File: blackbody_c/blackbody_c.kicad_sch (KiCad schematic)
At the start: 6 parts

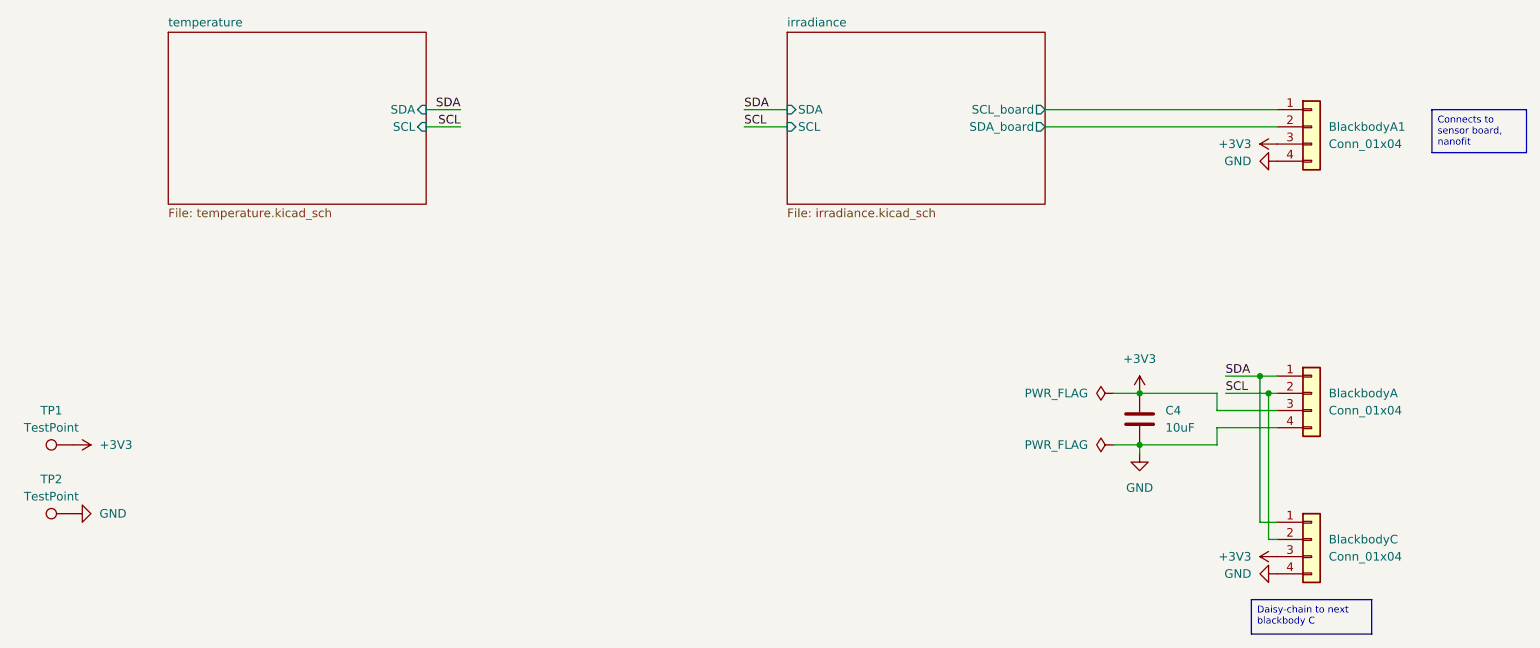
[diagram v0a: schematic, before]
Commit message: layout iteration 1
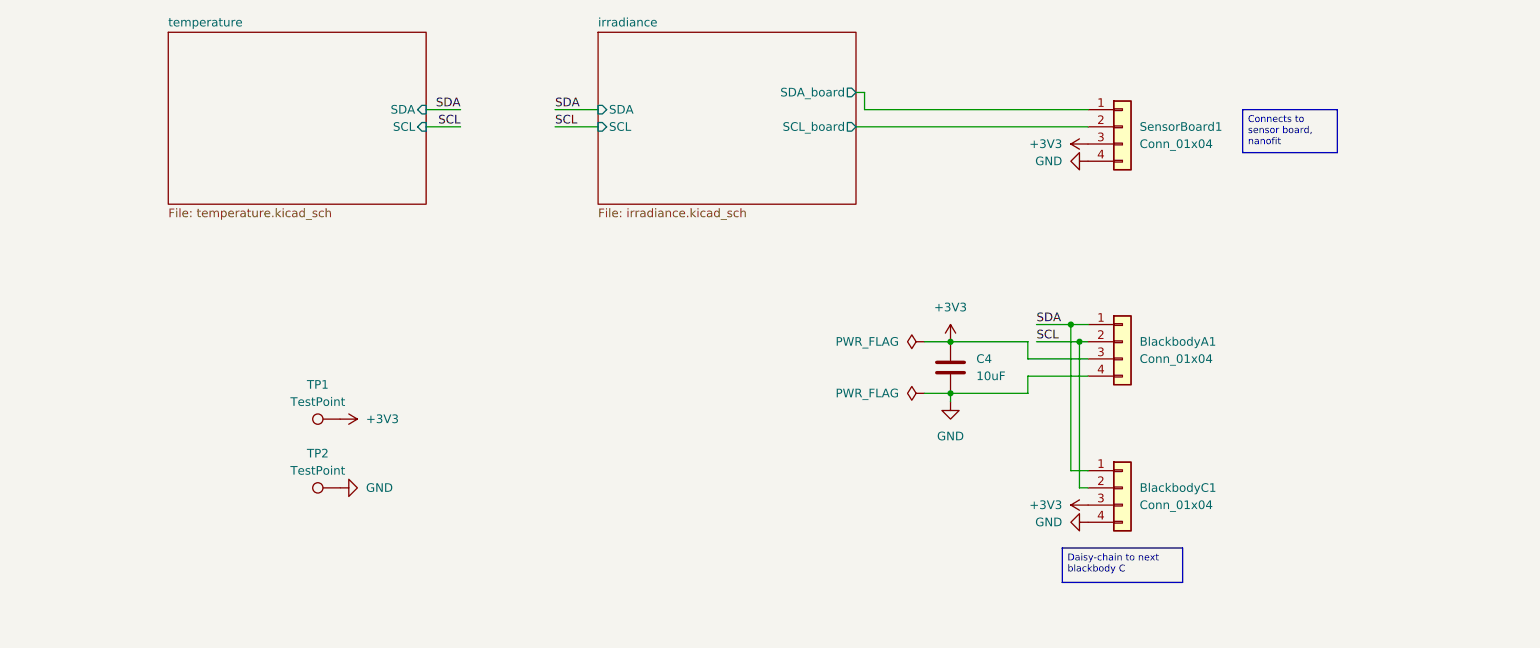
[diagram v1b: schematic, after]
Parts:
- BlackbodyA1: renamed from BlackbodyA; footprint (none) -> Blackbodies:MOLEX_1053091104
- BlackbodyC1: renamed from BlackbodyC; footprint (none) -> Blackbodies:MOLEX_1053091104
- C4: footprint (none) -> Capacitor_SMD:C_0805_2012Metric
- SensorBoard1: renamed from BlackbodyA1; footprint (none) -> Blackbodies:CONN_SD-105310-100_04_MOL
- TP1, TP2: footprint (none) -> UTSVT_Special:TestPoint_HEX_3mmID
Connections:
- net irradiance/SCL_board: now also SensorBoard1.2 (Pin_2); no longer SensorBoard1.1 (Pin_1)
- net irradiance/SDA_board: now also SensorBoard1.1 (Pin_1); no longer SensorBoard1.2 (Pin_2)
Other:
- moved on the sheet: BlackbodyA1, BlackbodyC1, C4, SensorBoard1, TP1, TP2
